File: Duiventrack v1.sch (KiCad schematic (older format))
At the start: 25 parts, among them P1 CONN_01X07, P2 CONN_01X02, U1 MCP1711-SOT23-5, U2 SP-ABZ-G

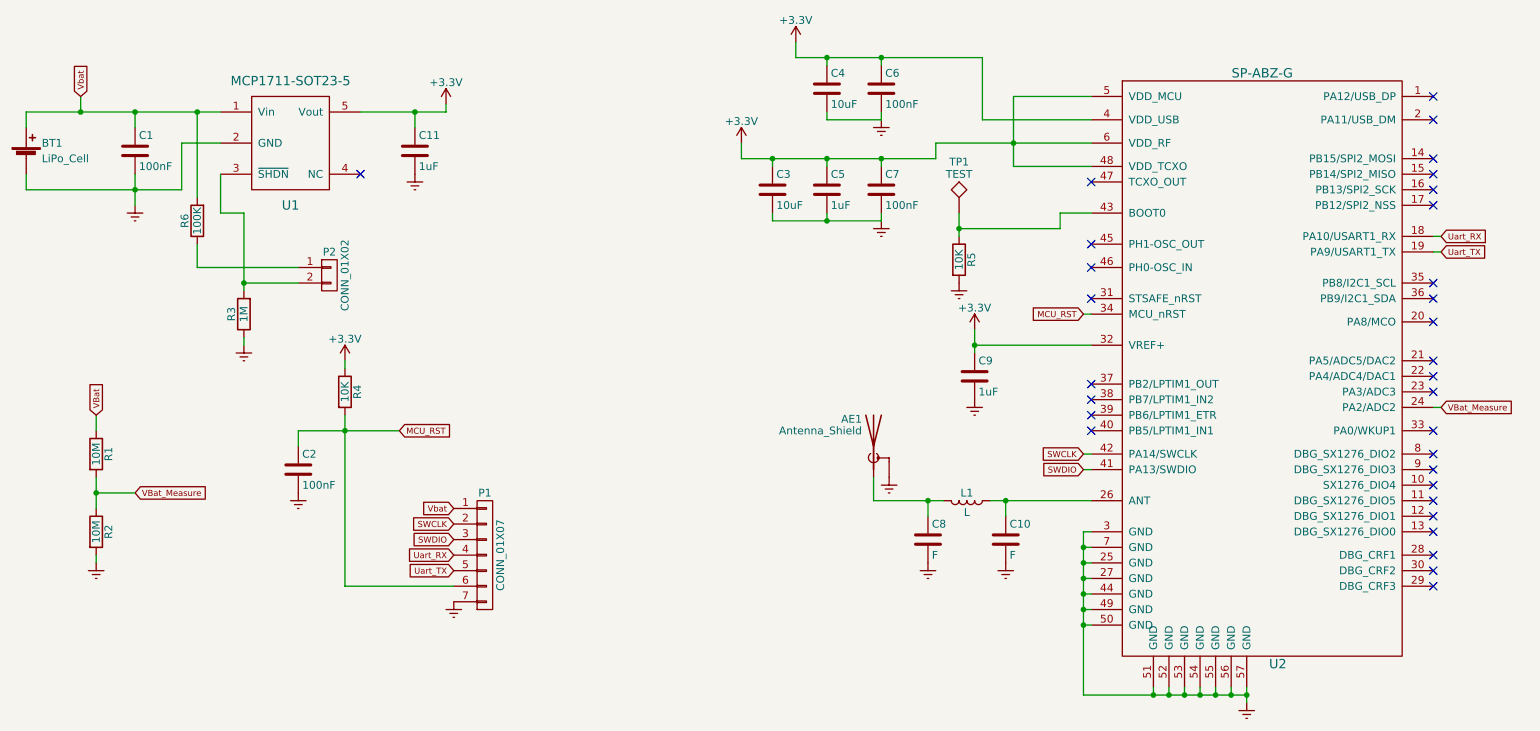
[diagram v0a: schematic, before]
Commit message: Crystal toegevoegd
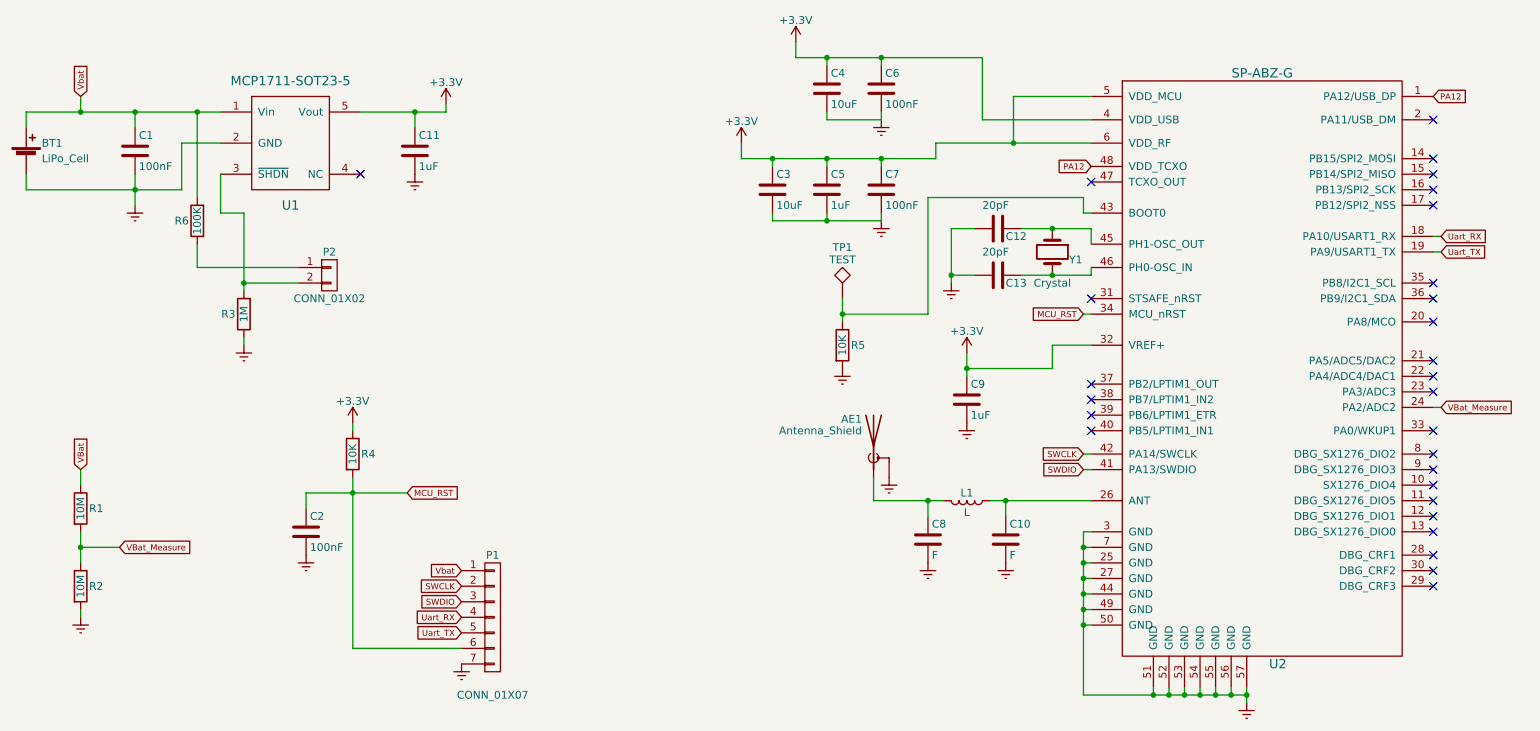
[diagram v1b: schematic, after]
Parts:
- added C12, C13: 20pF, Capacitors_SMD:C_0402, symbol C
- added Y1: Crystal, Crystals:Crystal_SMD_5032-2pin_5.0x3.2mm, symbol Crystal
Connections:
- net +3V3: no longer U2.48 (VDD_TCXO)
- net Earth: now also C12.2, C13.2
- net PA12: now reaches U2.1 (PA12/USB_DP)
- net PA12: now also U2.48 (VDD_TCXO)
- net at U2.45 (PH1-OSC_OUT): now also C12.1, Y1.1
- net at U2.46 (PH0-OSC_IN): now also C13.1, Y1.2
- no-connect marks 31 -> 28
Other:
- moved on the sheet: C2, C9, P1, R1, R2, R4, R5, TP1

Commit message: Revert "Crystal toegevoegd"
This reverts commit 51f246dfdab6a70a9bd41b0f28c72966c573f5f4.
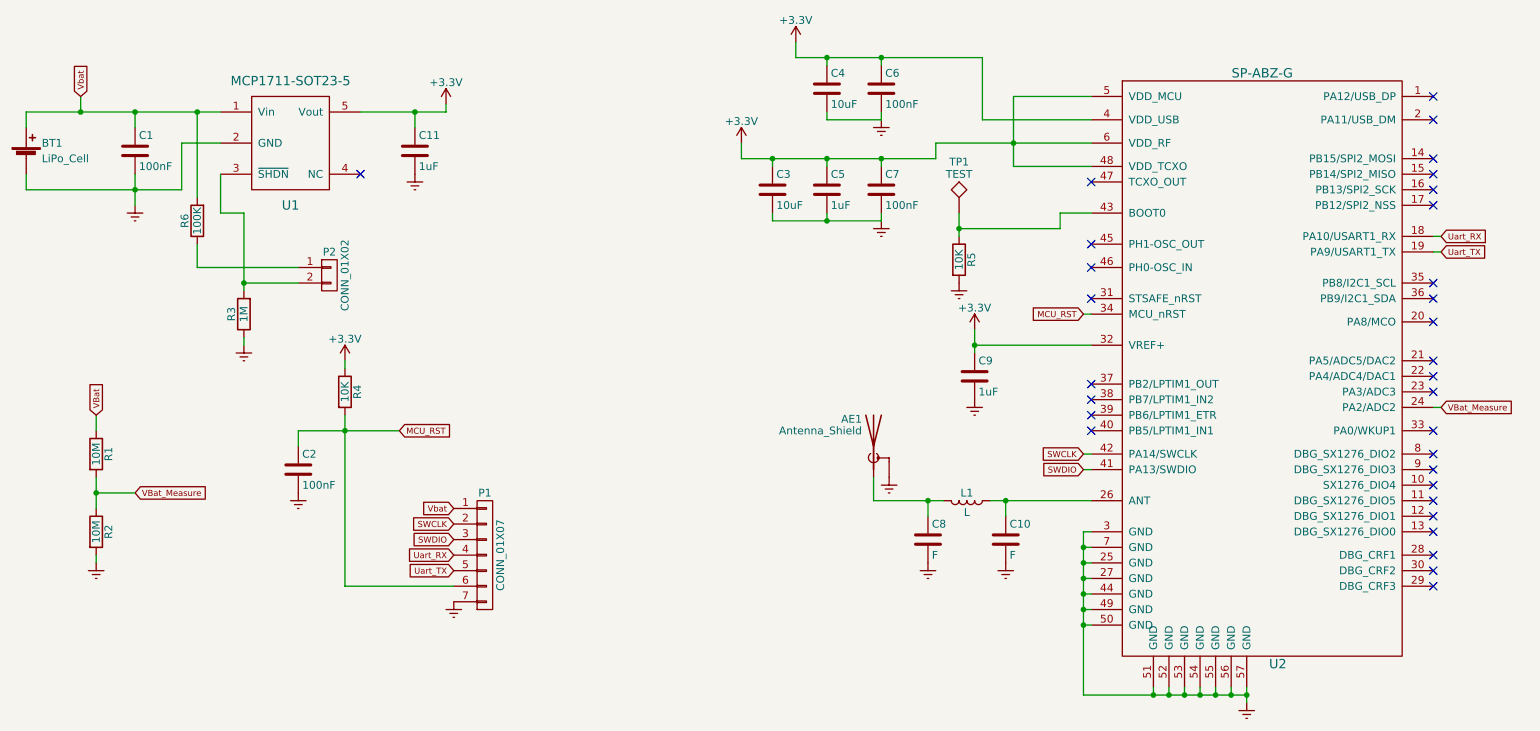
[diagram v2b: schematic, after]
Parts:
- removed C12, C13: 20pF, Capacitors_SMD:C_0402, symbol C
- removed Y1: Crystal, Crystals:Crystal_SMD_5032-2pin_5.0x3.2mm, symbol Crystal
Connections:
- net +3V3: now also U2.48 (VDD_TCXO)
- net PA12: no longer names the net of U2.1 (PA12/USB_DP)
- net PA12: no longer U2.48 (VDD_TCXO)
- no-connect marks 28 -> 31
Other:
- moved on the sheet: C2, C9, P1, R1, R2, R4, R5, TP1
